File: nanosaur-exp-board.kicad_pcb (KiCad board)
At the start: 2 copper layers, 80 x 20 mm, 21 parts, among them J1 jetson_nano, J2 Screw_Terminal_01x02, J3 Conn_i2c_oled, J4 Conn_i2c_oled, J5 Conn_motors, J6 Conn_buttons, J7 Conn_01x04, SW1 SW_SPDT

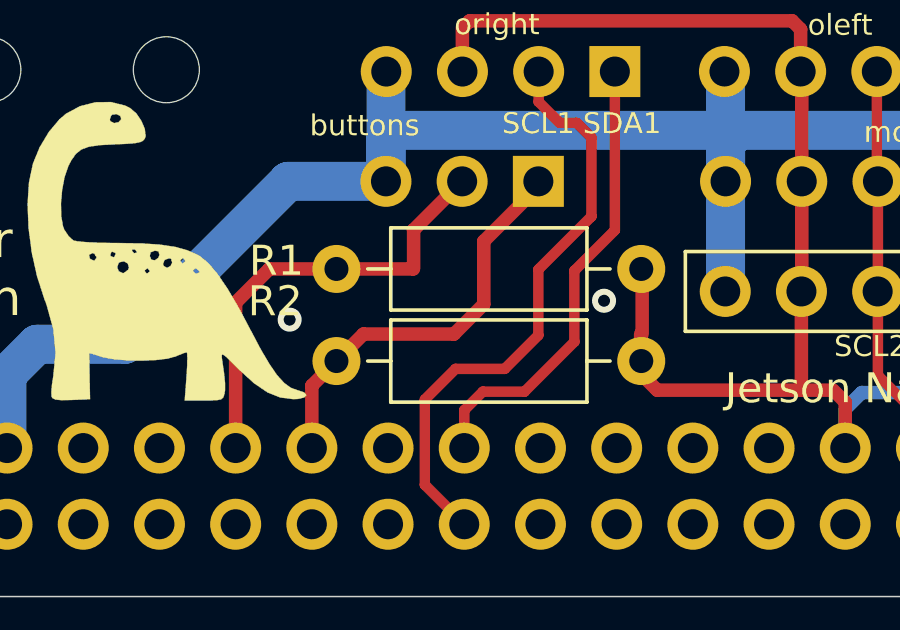
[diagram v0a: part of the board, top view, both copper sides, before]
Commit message: Fix DRC
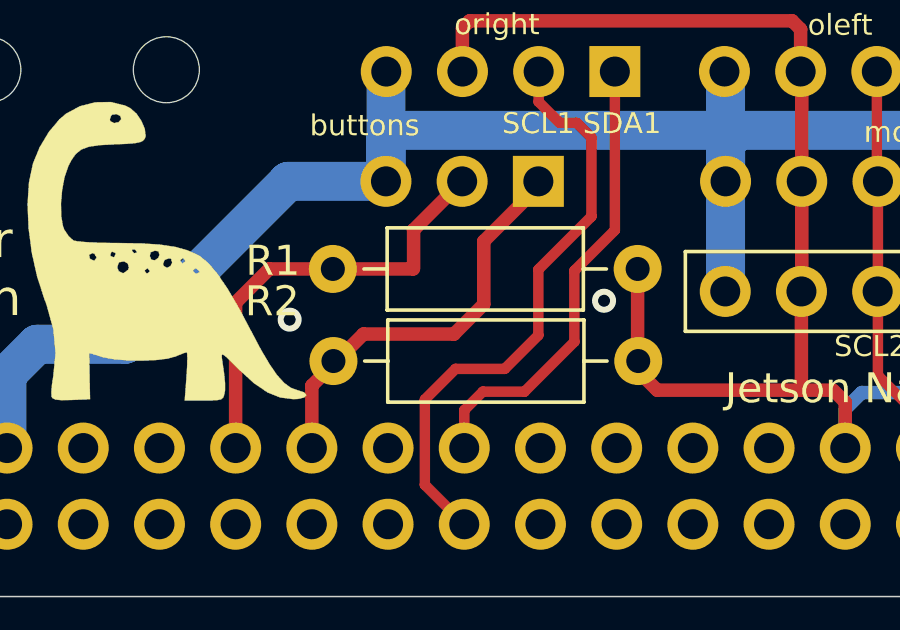
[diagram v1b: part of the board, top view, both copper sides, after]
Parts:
- moved R1 0.12 mm to (136.9, 92.4)
- moved R2 0.10 mm to (137.0, 95.5)
